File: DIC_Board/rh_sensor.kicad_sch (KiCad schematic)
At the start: 0 parts

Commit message: Wrapping up schematic
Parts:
- added J6: Conn_01x04, symbol Connector_Generic:Conn_01x04
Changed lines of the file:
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@@
 	(generator_version "10.0")
 	(paper "A4")
+	(symbol
+		(lib_id "Connector_Generic:Conn_01x04")
+		(at 218.44 86.36 0)
+		(unit 1)
+		(body_style 1)
+		(exclude_from_sim no)
+		(in_bom yes)
+		(on_board yes)
+		(in_pos_files yes)
+		(dnp no)
+		(fields_autoplaced yes)
+		(property "Reference" "J6"
+			(at 220.98 86.3599 0)
+			(show_name no)
+			(do_not_autoplace no)
+			(effects
+				(font
+					(size 1.27 1.27)
+				)
+				(justify left)
+			)
+		)
+		(property "Value" "Conn_01x04"
+			(at 220.98 88.8999 0)
+			(show_name no)
+			(do_not_autoplace no)
+			(effects
+				(font
+					(size 1.27 1.27)
+				)
+				(justify left)
+			)
+		)
+		(property "Footprint" ""
+			(at 218.44 86.36 0)
+			(hide yes)
+			(show_name no)
+			(do_not_autoplace no)
+			(effects
+				(font
+					(size 1.27 1.27)
+				)
+			)
+		)
+		(property "Datasheet" ""
+			(at 218.44 86.36 0)
+			(hide yes)
+			(show_name no)
+			(do_not_autoplace no)
+			(effects
+				(font
+					(size 1.27 1.27)
+				)
+			)
+		)
+		(property "Description" "Generic connector, single row, 01x04, script generated (kicad-library-utils/schlib/autogen/connector/)"
+			(at 218.44 86.36 0)
+			(hide yes)
+			(show_name no)
+			(do_not_autoplace no)
+			(effects
+				(font
+					(size 1.27 1.27)
+				)
+			)
+		)
+		(pin "1"
+		)
+		(pin "4"
+		)
+		(pin "3"
+		)
+		(pin "2"
+		)
+		(instances
+			(project "DIC_Board"
+				(path "/bb0ef0df-c181-443a-843c-695cd2e0efee/15388a04-aea8-414b-8903-58a719a8054d/a18bb969-316f-4822-a8ba-f772f1045bbc"
+					(reference "J6")
+					(unit 1)
+				)
+			)
+		)
+	)
 )

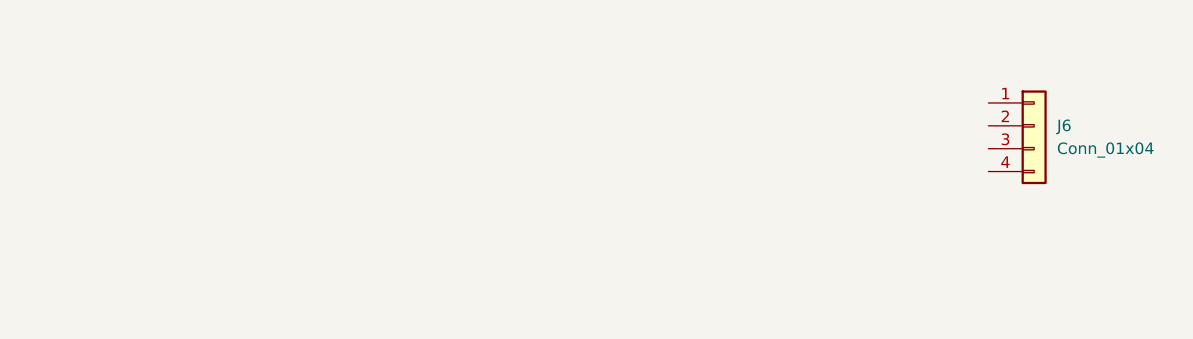
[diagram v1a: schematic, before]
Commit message: Checkpoint current schematic state
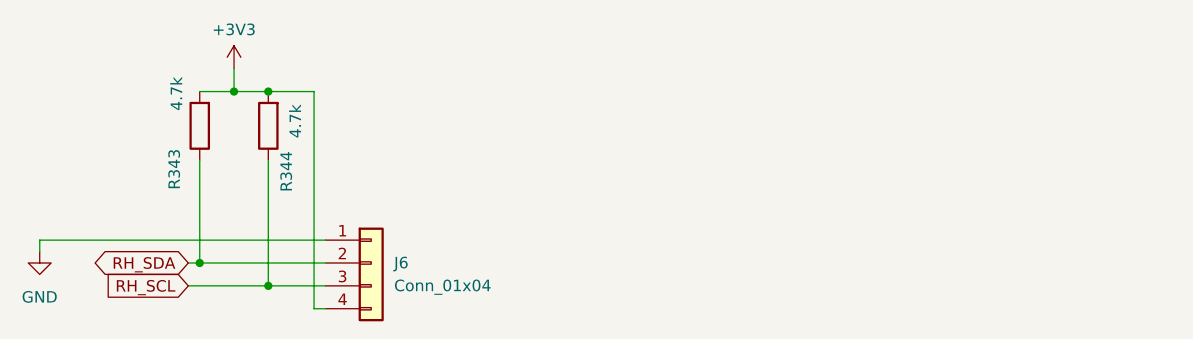
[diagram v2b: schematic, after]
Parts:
- added R343, R344: 4.7k, symbol Device:R
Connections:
- net GND: now reaches J6.1 (Pin_1)
- net RH_SDA: now reaches J6.2 (Pin_2)
- net RH_SDA: now also R343.1
- net RH_SCL: now reaches J6.3 (Pin_3)
- net RH_SCL: now also R344.1
- net +3V3: now reaches J6.4 (Pin_4)
- net +3V3: now also R343.2, R344.2
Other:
- moved on the sheet: J6
